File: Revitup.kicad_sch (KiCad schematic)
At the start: 8 parts, among them J2 Screw_Terminal_01x03, Q1 BC548, U1 ESP32-C6-MINI-1

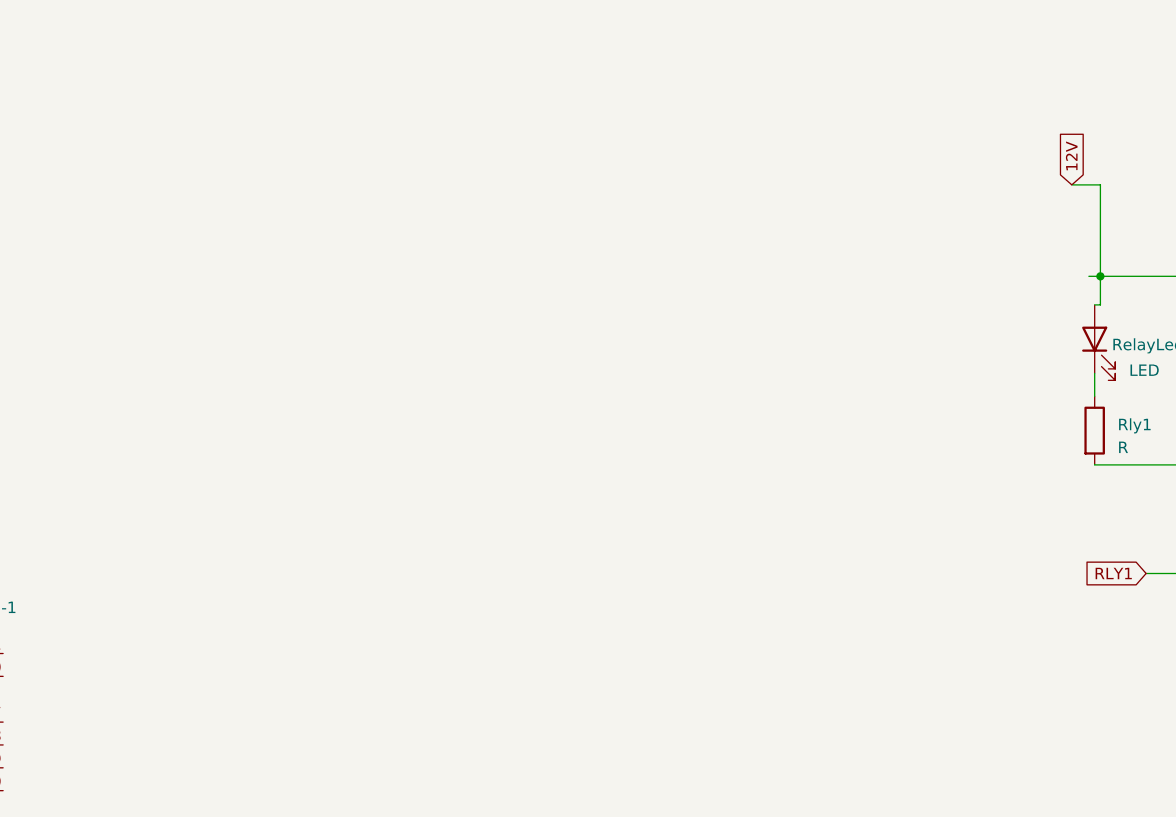
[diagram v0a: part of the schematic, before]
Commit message: Relays
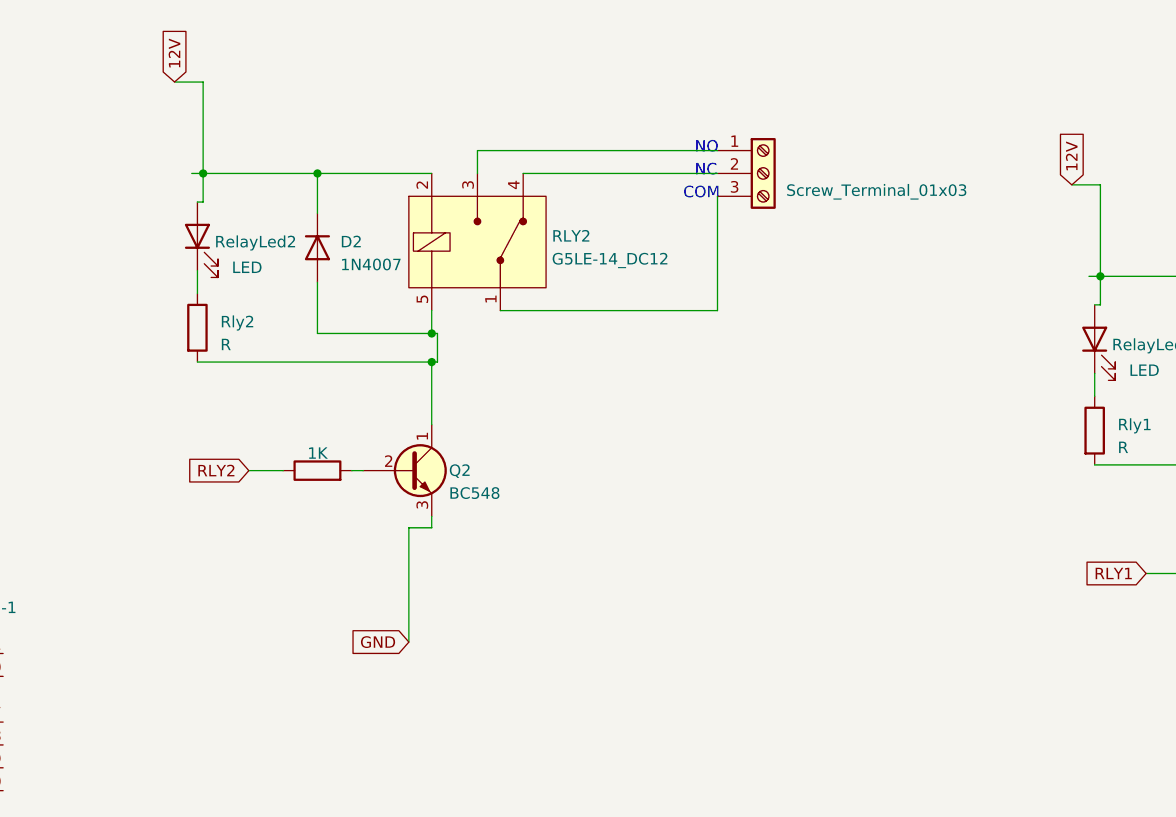
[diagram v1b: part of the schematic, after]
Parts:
- added D2: 1N4007, Diode_THT:D_DO-41_SOD81_P10.16mm_Horizontal, symbol Diode:1N4007
- added J1: Screw_Terminal_01x03, TerminalBlock_Phoenix:TerminalBlock_Phoenix_MKDS-1,5-3_1x03_P5.00mm_Horizontal, symbol Connector:Screw_Terminal_01x03
- added Q2: BC548, Package_TO_SOT_THT:TO-92_Inline_Wide, symbol PCM_Transistor_BJT_AKL:BC548
- added R2: 1K, Resistor_SMD:R_0805_2012Metric_Pad1.20x1.40mm_HandSolder, symbol Device:R
- added RLY2: G5LE-14_DC12, digikey-footprints:Relay_THT_G5LE-14, symbol dk_Power-Relays-Over-2-Amps:G5LE-14_DC12
- added RelayLed2: LED, LED_SMD:LED_1206_3216Metric_Pad1.42x1.75mm_HandSolder, symbol Device:LED
- added Rly2: R, Resistor_SMD:R_1206_3216Metric_Pad1.30x1.75mm_HandSolder, symbol Device:R
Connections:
- net 12V: now also D2.1 (K), RLY2.2 (COIL), RelayLed2.2 (A)
- net GND: now also Q2.3 (E)
- new net: D2.2 (A), Q2.1 (C), RLY2.5 (COIL), Rly2.2
- new net: Q2.2 (B), R2.2
- new net: RelayLed2.1 (K), Rly2.1
- new net: J1.3 (Pin_3), RLY2.1 (COM)
- new net: J1.1 (Pin_1), RLY2.3 (NO)
- new net: J1.2 (Pin_2), RLY2.4 (NC)
- new net RLY2: R2.1
